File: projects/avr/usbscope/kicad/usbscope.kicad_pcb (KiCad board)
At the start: 2 copper layers, 50.8 x 27.9 mm, 17 parts, among them J1 USB_2, P1 CONN_1, P2 CONN_1, P3 CONN_1, P4 CONN_6, P5 CONN_1, U1 ATTINY45-20PU

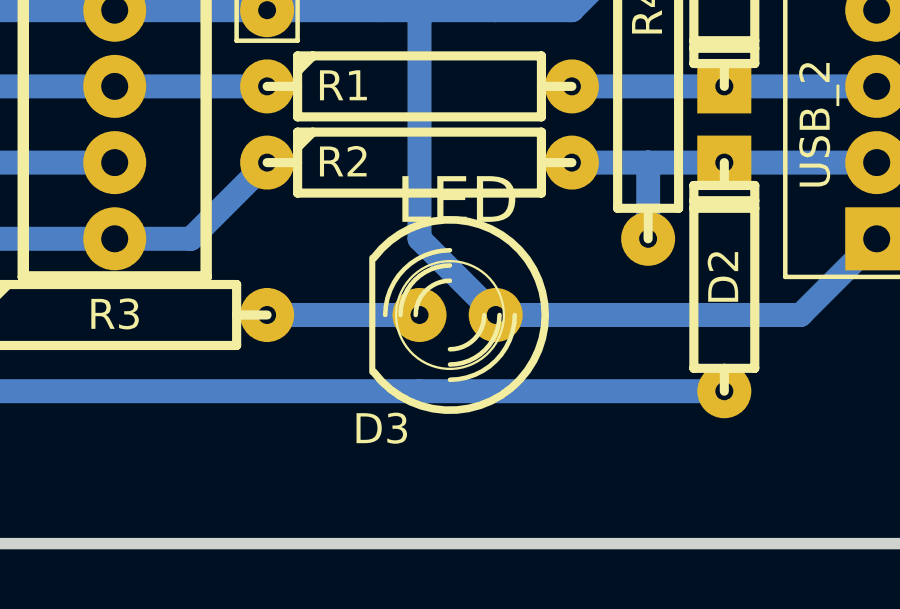
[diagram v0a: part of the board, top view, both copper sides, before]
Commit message: update kicad files
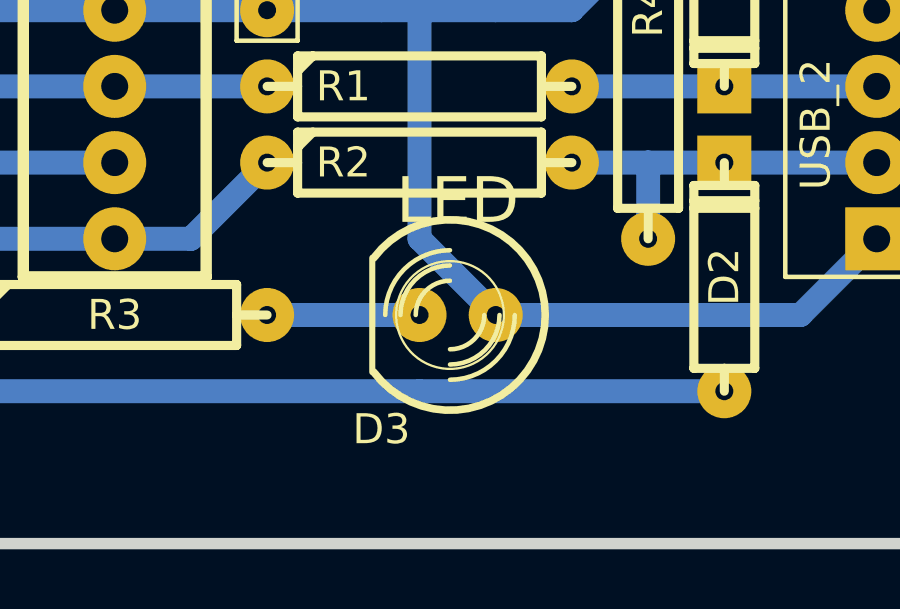
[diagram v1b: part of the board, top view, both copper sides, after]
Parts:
- C1: footprint kicad:C2 -> common:C2
- C2: footprint kicad:CP_5x11mm -> common:CP_5x11mm
- D1, D2: footprint kicad:D3 -> common:D3
- D3: footprint kicad:LED-5MM -> common:LED-5MM
- J1: footprint kicad:USB4 -> common:USB4
- P1, P2, P3, P5: footprint kicad:PIN_ARRAY_1X1 -> common:PIN_ARRAY_1X1
- P4: footprint kicad:PIN_ARRAY_6X1 -> common:PIN_ARRAY_6X1
- R1, R2, R3, R4, R5: footprint kicad:R4 -> common:R4
- U1: footprint kicad:DIP-8__300 -> common:DIP-8__300
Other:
- net class Default removed
